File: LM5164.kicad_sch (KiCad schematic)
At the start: 11 parts, among them U8 ME6118A33, U9 LM5164DDA

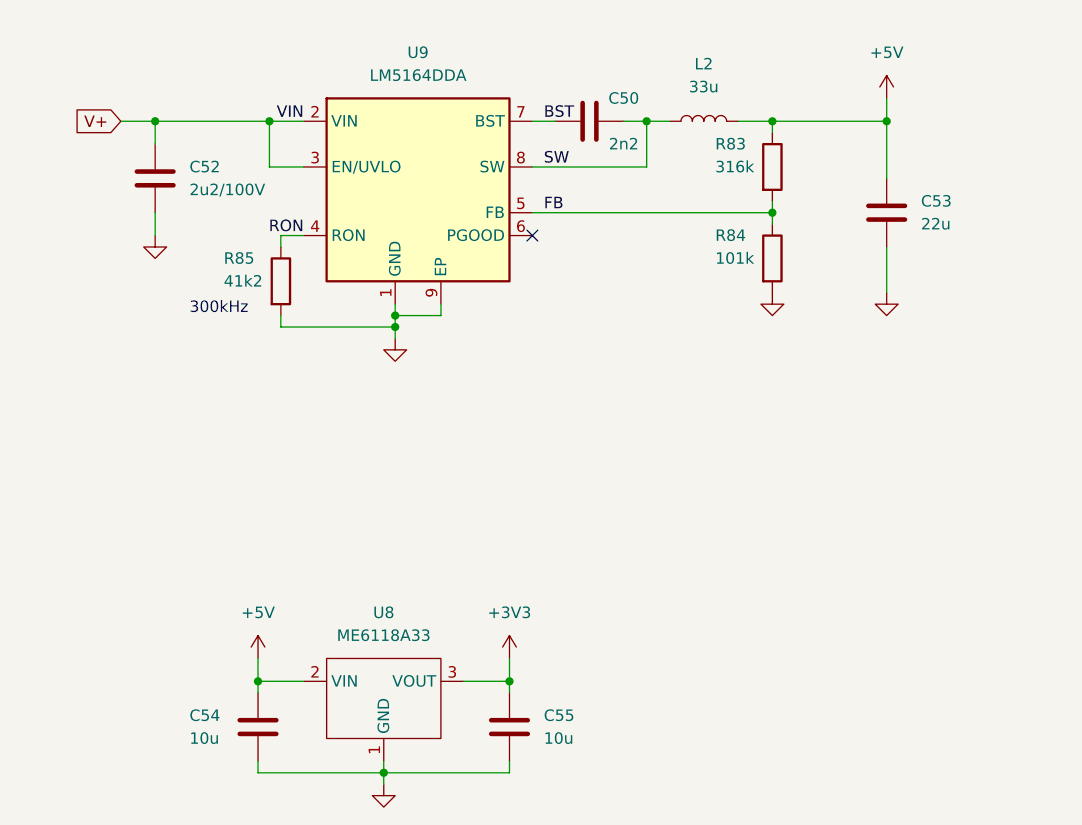
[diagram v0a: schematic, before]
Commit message: almost ready to order
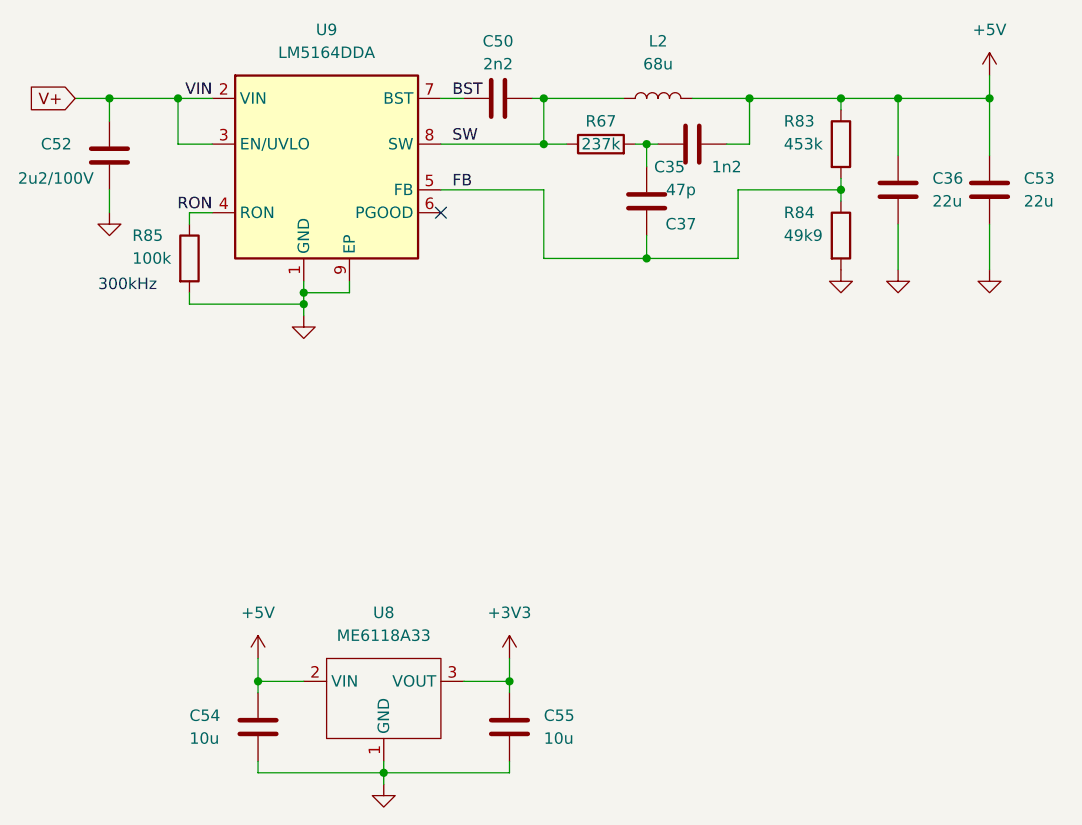
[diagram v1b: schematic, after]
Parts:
- added C35: 1n2, Capacitor_SMD:C_0603_1608Metric, symbol Device:C
- added C36: 22u, Capacitor_SMD:C_0805_2012Metric, symbol Device:C
- added C37: 47p, Capacitor_SMD:C_0805_2012Metric, symbol Device:C
- added R67: 237k, Resistor_SMD:R_0805_2012Metric, symbol Device:R
- C50: footprint Capacitor_SMD:C_0805_2012Metric -> Capacitor_SMD:C_0603_1608Metric
- C53: footprint Capacitor_SMD:C_1210_3225Metric -> Capacitor_SMD:C_0805_2012Metric
- L2: value 33u -> 68u; LCSC C206300 -> C206245
- R83: value 316k -> 453k
- R84: value 101k -> 49k9; LCSC C114540 -> (none)
- R85: value 41k2 -> 100k
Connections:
- net +5V: now also C35.2, C36.1
- net FB: now also C37.1
- net GND: now also C36.2
- net SW: now also R67.1
- new net: C35.1, C37.2, R67.2
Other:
- moved on the sheet: C50, C52, C53, L2, R83, R84, R85, U9
